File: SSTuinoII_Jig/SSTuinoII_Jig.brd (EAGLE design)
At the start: 73.6 x 73.3 mm, 13 parts, among them J1 MuseLab CMSIS-DAP, Q1 BS170

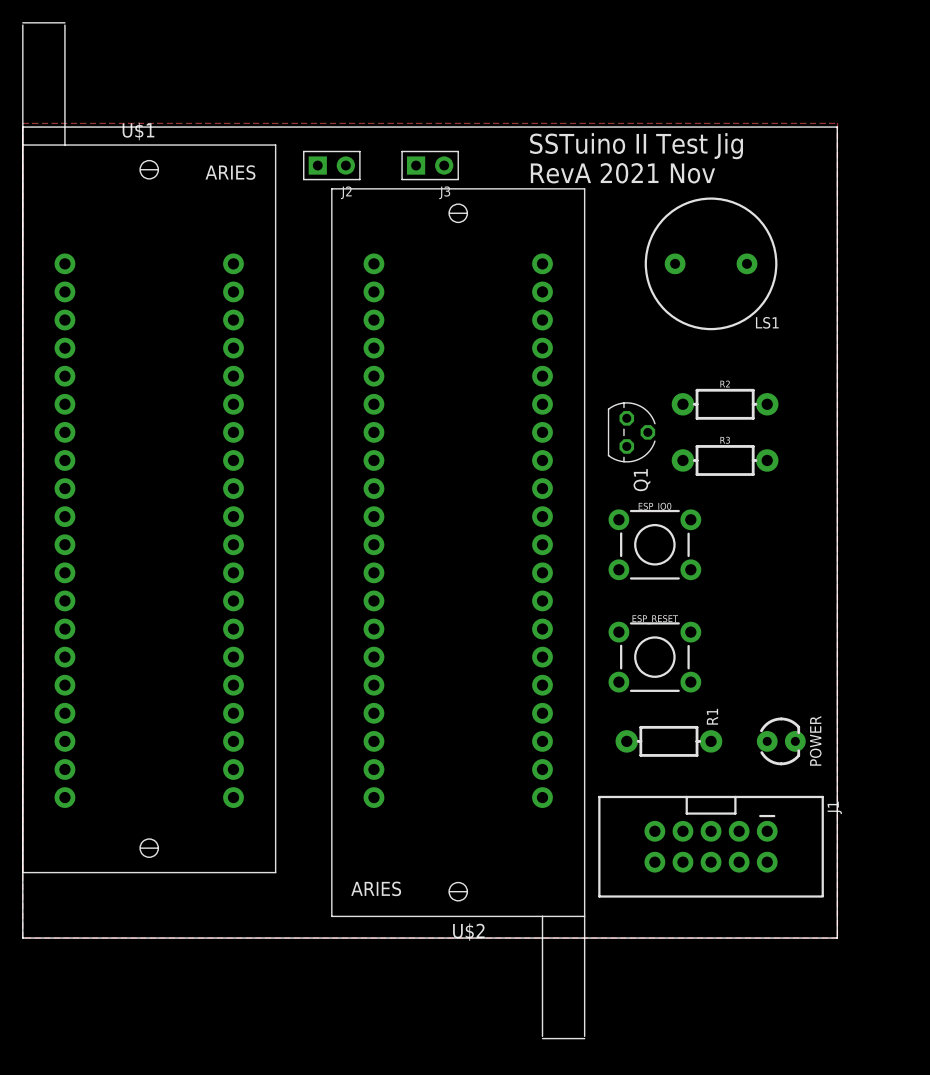
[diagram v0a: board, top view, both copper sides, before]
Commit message: finalised test jig
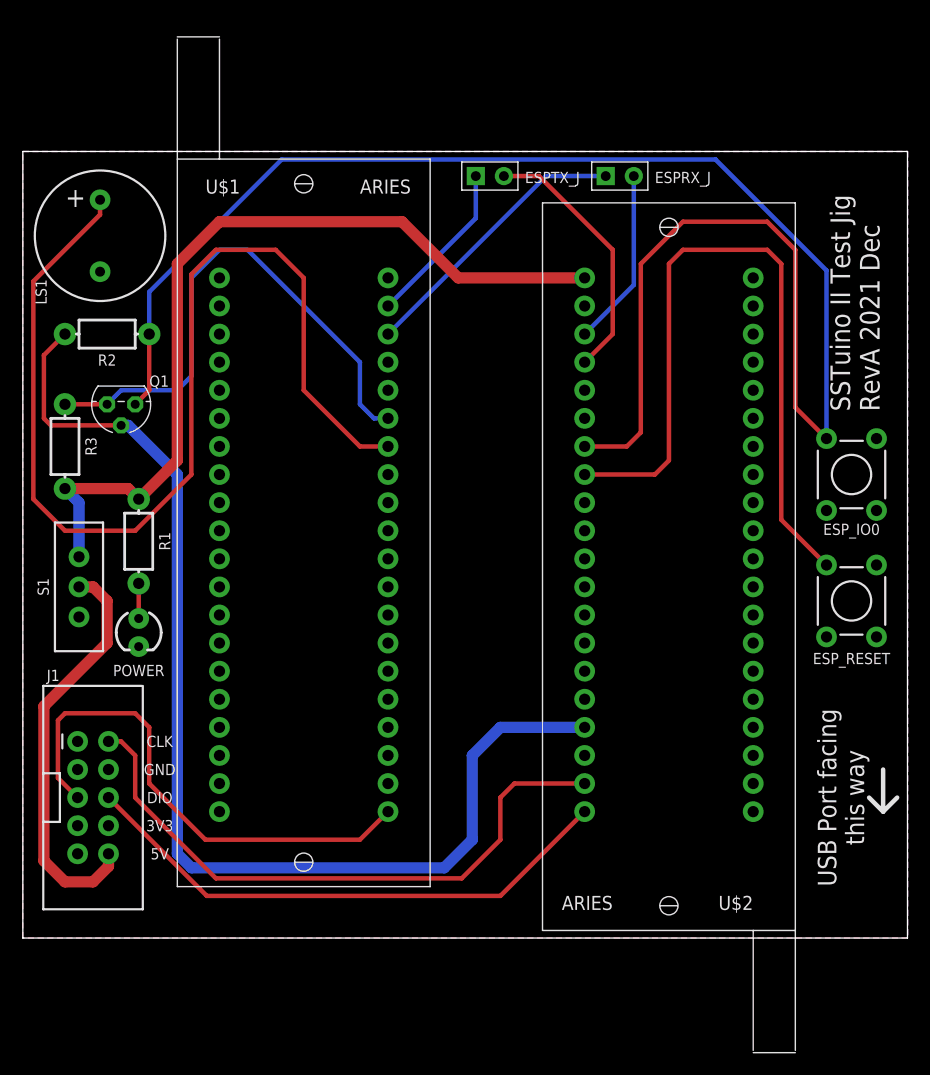
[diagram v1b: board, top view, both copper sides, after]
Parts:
- removed J2, J3: (no value), OPL_Connector:H2-2.54
- added ESPRX_J, ESPTX_J: (no value), OPL_Connector:H2-2.54
- added S1: (no value), SparkFun-Switches:SWITCH_SPDT_PTH_11.6X4.0MM_KIT
- J1: value MuseLab CMSIS-DAP -> MuseLab CMSIS-DAP Only
- moved R3 59.7 mm to (3.81, 44.5), turned to 270 degrees
- moved POWER 58.9 mm to (10.5, 27.6), turned to 270 degrees
- moved R2 56.2 mm to (7.62, 54.6), turned to 180 degrees
- moved J1 56.1 mm to (6.35, 12.7), turned to 0 degrees
- moved LS1 55.3 mm to (6.99, 63.5), turned to 90 degrees
- moved R1 51.2 mm to (10.5, 35.9), turned to 90 degrees
- moved Q1 45.8 mm to (8.89, 48.3), turned to 180 degrees
- moved U$2 19.1 mm to (66.0, 11.4)
- moved ESP_IO0 18.9 mm to (74.9, 41.9), turned to 270 degrees
- moved ESP_RESET 18.5 mm to (74.9, 30.5), turned to 270 degrees
- moved U$1 14.0 mm to (17.8, 59.7)
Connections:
- new net PWR: J1.10, S1.2
- net 5V: now also S1.1; no longer J1.10
- net ESP_RX: now also ESPRX_J.2; no longer J3.2
- net ESP_TX: now also ESPTX_J.2; no longer J2.2
- net GND: now also U$1.P$25
- net MEGA_RX: now also ESPTX_J.1; no longer J2.1
- net MEGA_TX: now also ESPRX_J.1; no longer J3.1
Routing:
- net ESP_IO0: track 0.00 -> 151.9 mm
- net 3.3V: track 0.00 -> 103.9 mm
- net MEGA_D5: track 0.00 -> 97.3 mm
- net 5V: track 0.00 -> 77.0 mm
- net ESP_EN: track 0.00 -> 66.1 mm
- net SWCLK: track 0.00 -> 56.2 mm
- net SWDIO: track 0.00 -> 49.9 mm
- net MEGA_D4: track 0.00 -> 48.7 mm
- net NRST: track 0.00 -> 46.6 mm
- net PWR: track 0.00 -> 37.3 mm
- net MEGA_TX: track 0.00 -> 25.6 mm
- net ESP_TX: track 0.00 -> 23.8 mm
- net ESP_RX: track 0.00 -> 16.1 mm
- net MEGA_RX: track 0.00 -> 15.0 mm
- net N$1: track 0.00 -> 3.18 mm
- added copper zone on layer 16, net GND
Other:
- board size 73.6 x 73.3 mm -> 80 x 71.1 mm
- board text added: "+"
- board text added: "3V3"
- board text added: "5V"
- board text added: "CLK"
- board text added: "DIO"
- board text added: "GND"
- board text added: "SSTuino II Test Jig RevA 2021 Dec"
- board text added: "USB Port facing this way"
- board text removed: "SSTuino II Test Jig RevA 2021 Nov"
